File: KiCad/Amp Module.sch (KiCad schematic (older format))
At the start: 56 parts, among them J1 DSP, J2 LITEMOD, U1 NE5532, U2 NE5532, U3 TL072, U4 LM393, U5 74HC08, U6 TL072, U7 AMS1117-5.0

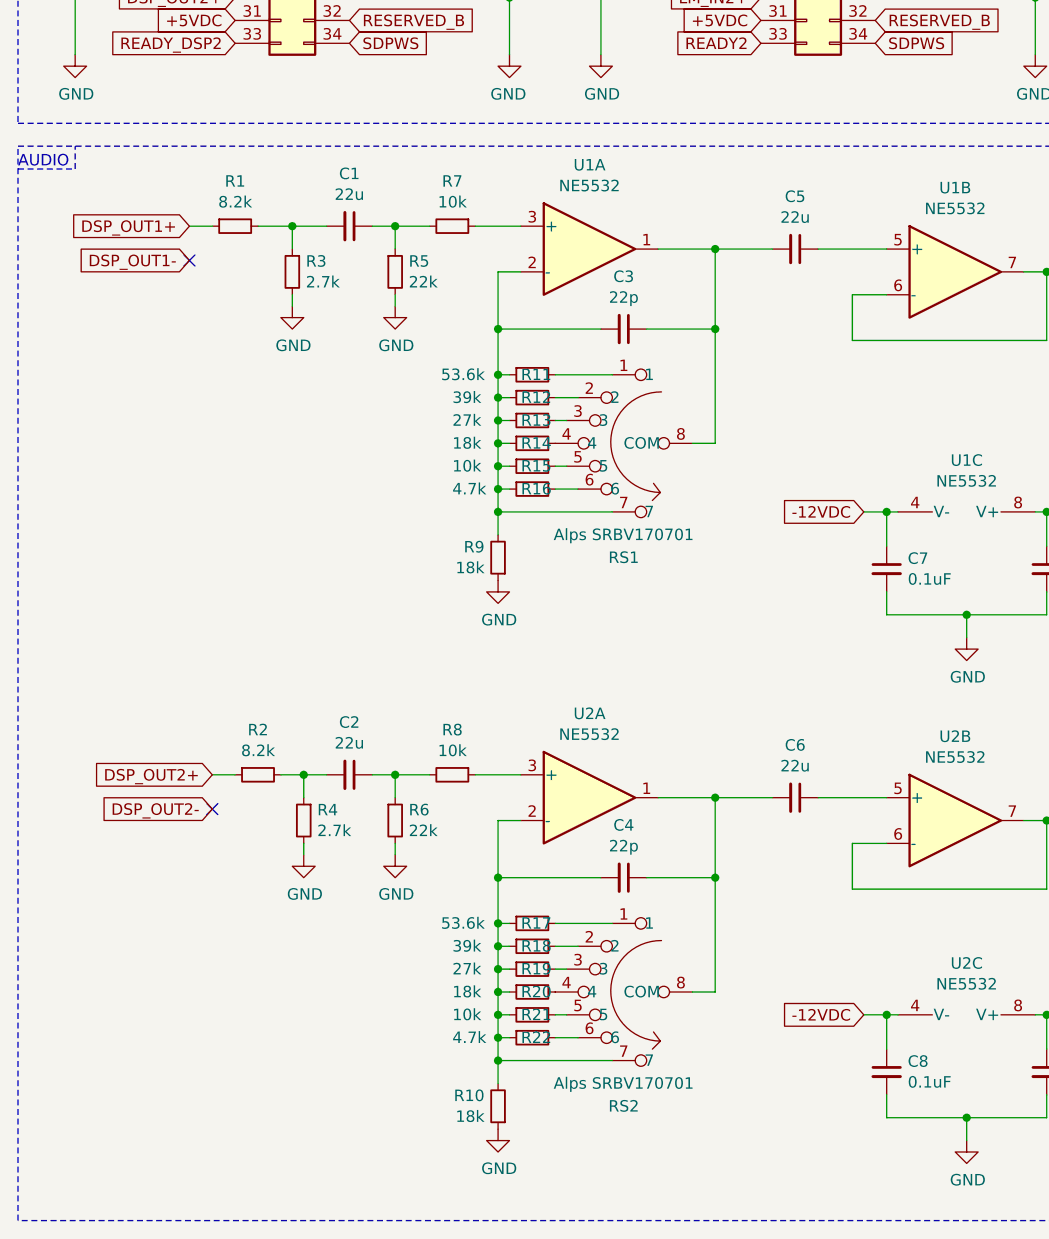
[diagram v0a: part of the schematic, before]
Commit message: edited chez Gabri's
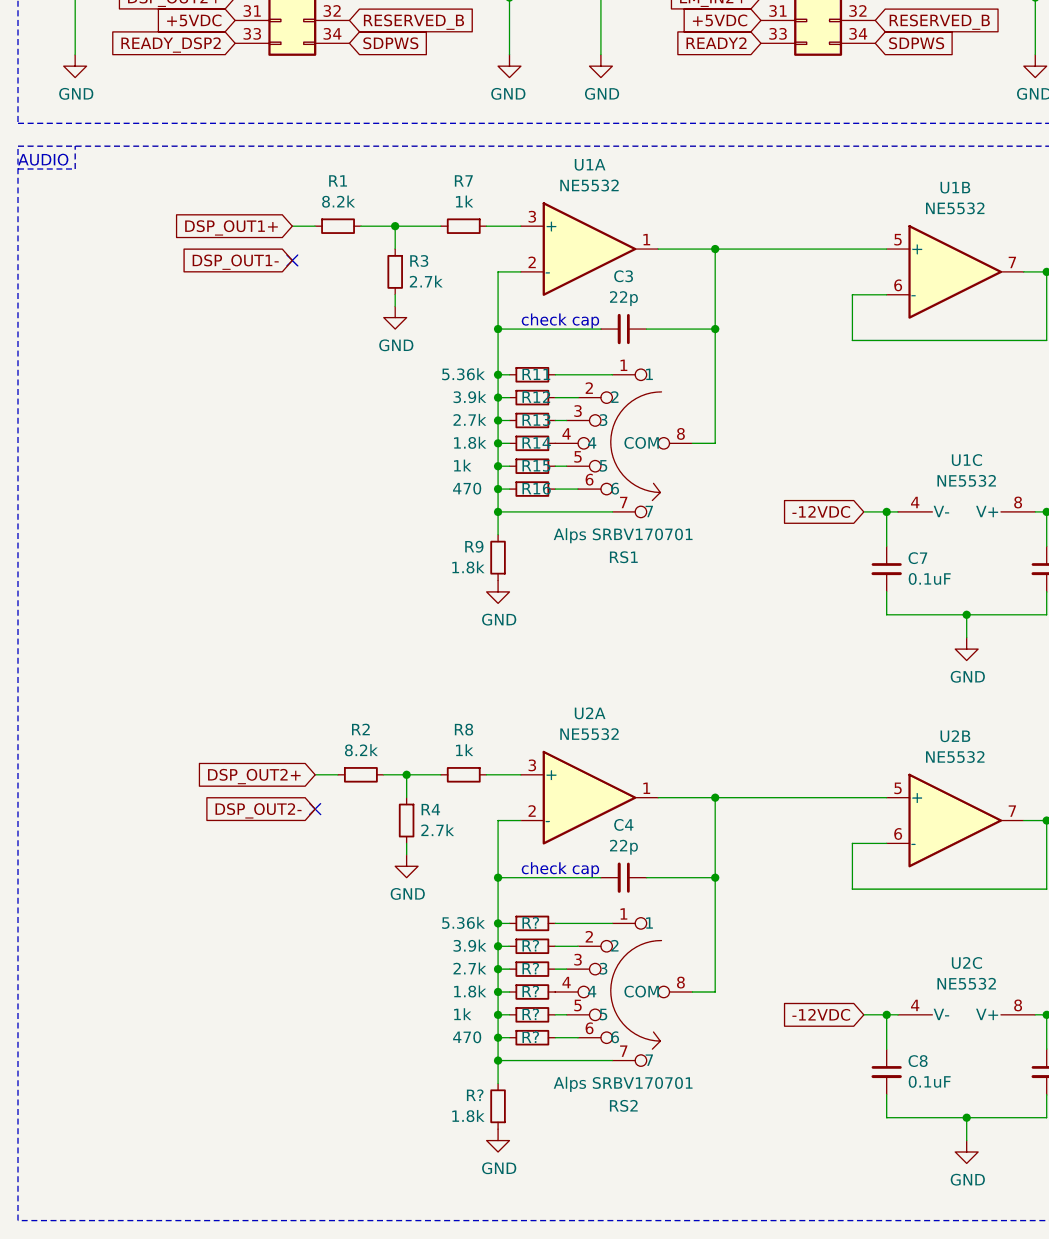
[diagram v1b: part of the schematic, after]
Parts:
- removed C1, C2, C5, C6: 22u, symbol Device:C_Small
- removed R10, R20: 18k, symbol Device:R_Small
- removed R17: 53.6k, symbol Device:R_Small
- removed R18: 39k, symbol Device:R_Small
- removed R19: 27k, symbol Device:R_Small
- removed R21: 10k, symbol Device:R_Small
- removed R22: 4.7k, symbol Device:R_Small
- removed R5, R6: 22k, symbol Device:R_Small
- added R? (x2): 1.8k, symbol Device:R_Small
- added R?: 1k, symbol Device:R_Small
- added R?: 2.7k, symbol Device:R_Small
- added R?: 3.9k, symbol Device:R_Small
- added R?: 5.36k, symbol Device:R_Small
- added R?: 470, symbol Device:R_Small
- R11: value 53.6k -> 5.36k
- R12: value 39k -> 3.9k
- R13: value 27k -> 2.7k
- R14, R9: value 18k -> 1.8k
- R15, R7, R8: value 10k -> 1k
- R16: value 4.7k -> 470
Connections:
- net GND: now also R?.1
- net at R1.2, R3.1: now also R7.2
- net at R2.2, R4.1: now also R8.2
- net at C3.1, RS1.8 (COM), U1.1: now also U1.5 (+)
- net at C4.1, RS2.8 (COM), U2.1: now also U2.5 (+)
- net at C4.2, RS2.7, U2.2 (-): now also R?.1, R?.1, R?.1, R?.1, R?.1, R?.1, R?.2
- net at RS2.1: now also R?.2
- net at RS2.2: now also R?.2
- net at RS2.3: now also R?.2
- net at RS2.4: now also R?.2
- net at RS2.5: now also R?.2
- net at RS2.6: now also R?.2
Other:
- note added: "check cap"
- moved on the sheet: R1, R2, R3, R4, R7, R8
